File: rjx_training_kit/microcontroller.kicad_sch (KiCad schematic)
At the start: 2 parts, among them SW2 SW_Push, U1 STM32F407VGTx

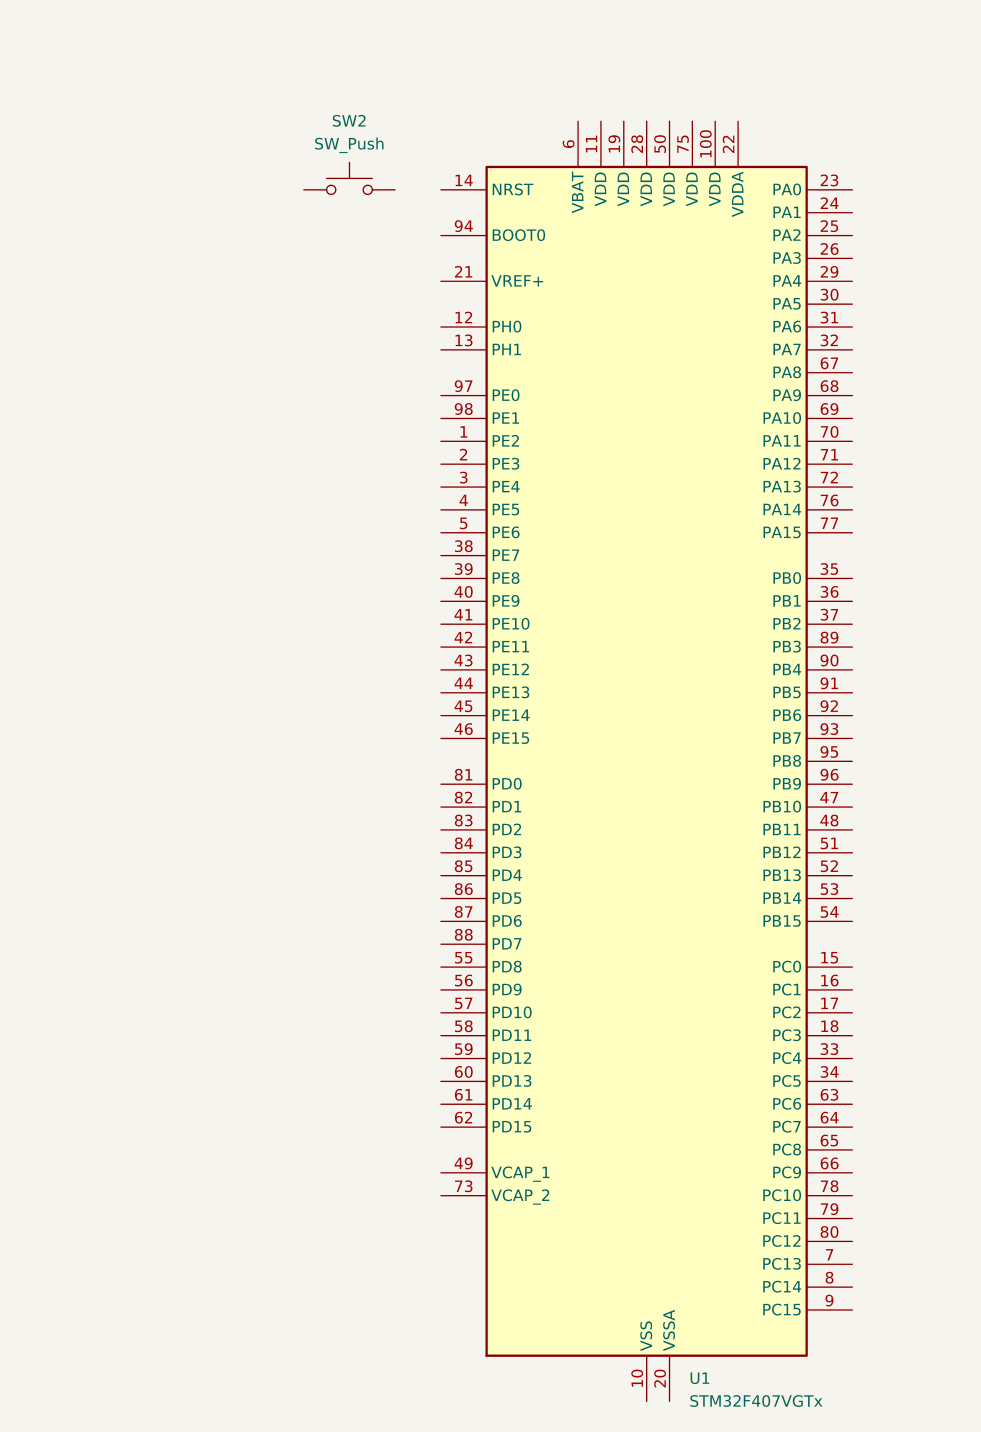
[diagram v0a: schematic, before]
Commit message: Update
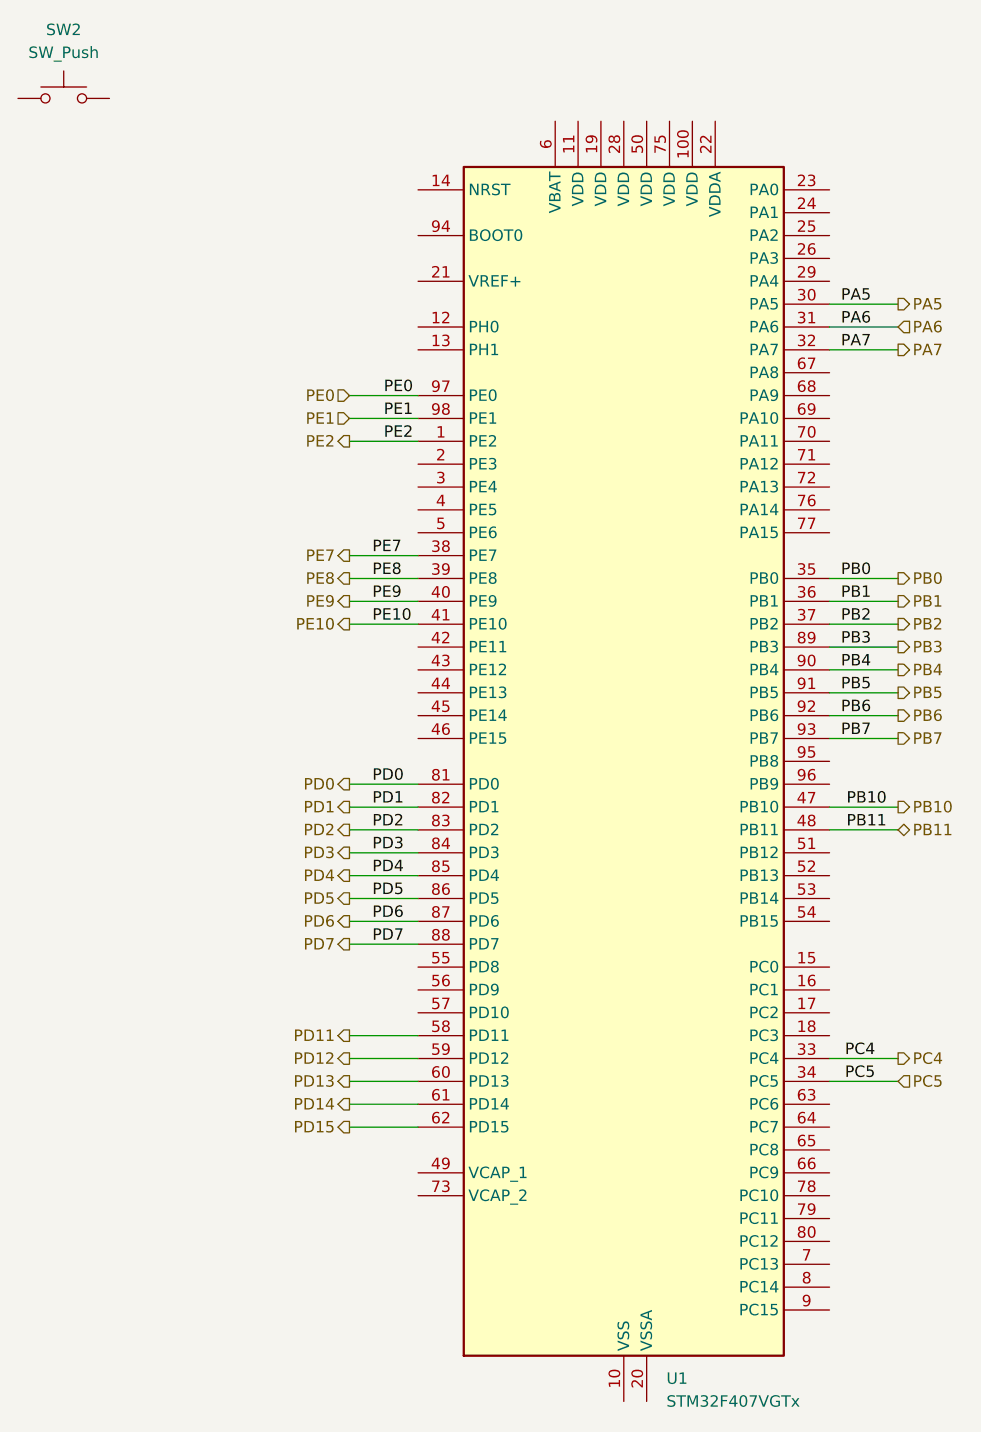
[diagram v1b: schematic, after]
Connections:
- net PE2: now reaches U1.1 (PE2)
- net PA5: now reaches U1.30 (PA5)
- net PA6: now reaches U1.31 (PA6)
- net PA7: now reaches U1.32 (PA7)
- net PC4: now reaches U1.33 (PC4)
- net PC5: now reaches U1.34 (PC5)
- net PB0: now reaches U1.35 (PB0)
- net PB1: now reaches U1.36 (PB1)
- net PB2: now reaches U1.37 (PB2)
- net PE7: now reaches U1.38 (PE7)
- net PE8: now reaches U1.39 (PE8)
- net PE9: now reaches U1.40 (PE9)
- net PE10: now reaches U1.41 (PE10)
- net PB10: now reaches U1.47 (PB10)
- net PB11: now reaches U1.48 (PB11)
- net PD11: now reaches U1.58 (PD11)
- net PD12: now reaches U1.59 (PD12)
- net PD13: now reaches U1.60 (PD13)
- net PD14: now reaches U1.61 (PD14)
- net PD15: now reaches U1.62 (PD15)
- net PD0: now reaches U1.81 (PD0)
- net PD1: now reaches U1.82 (PD1)
- net PD2: now reaches U1.83 (PD2)
- net PD3: now reaches U1.84 (PD3)
- net PD4: now reaches U1.85 (PD4)
- net PD5: now reaches U1.86 (PD5)
- net PD6: now reaches U1.87 (PD6)
- net PD7: now reaches U1.88 (PD7)
- net PB3: now reaches U1.89 (PB3)
- net PB4: now reaches U1.90 (PB4)
- net PB5: now reaches U1.91 (PB5)
- net PB6: now reaches U1.92 (PB6)
- net PB7: now reaches U1.93 (PB7)
- net PE0: now reaches U1.97 (PE0)
- net PE1: now reaches U1.98 (PE1)
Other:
- moved on the sheet: SW2, U1
